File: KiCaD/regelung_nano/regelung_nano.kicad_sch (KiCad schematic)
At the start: 3 parts

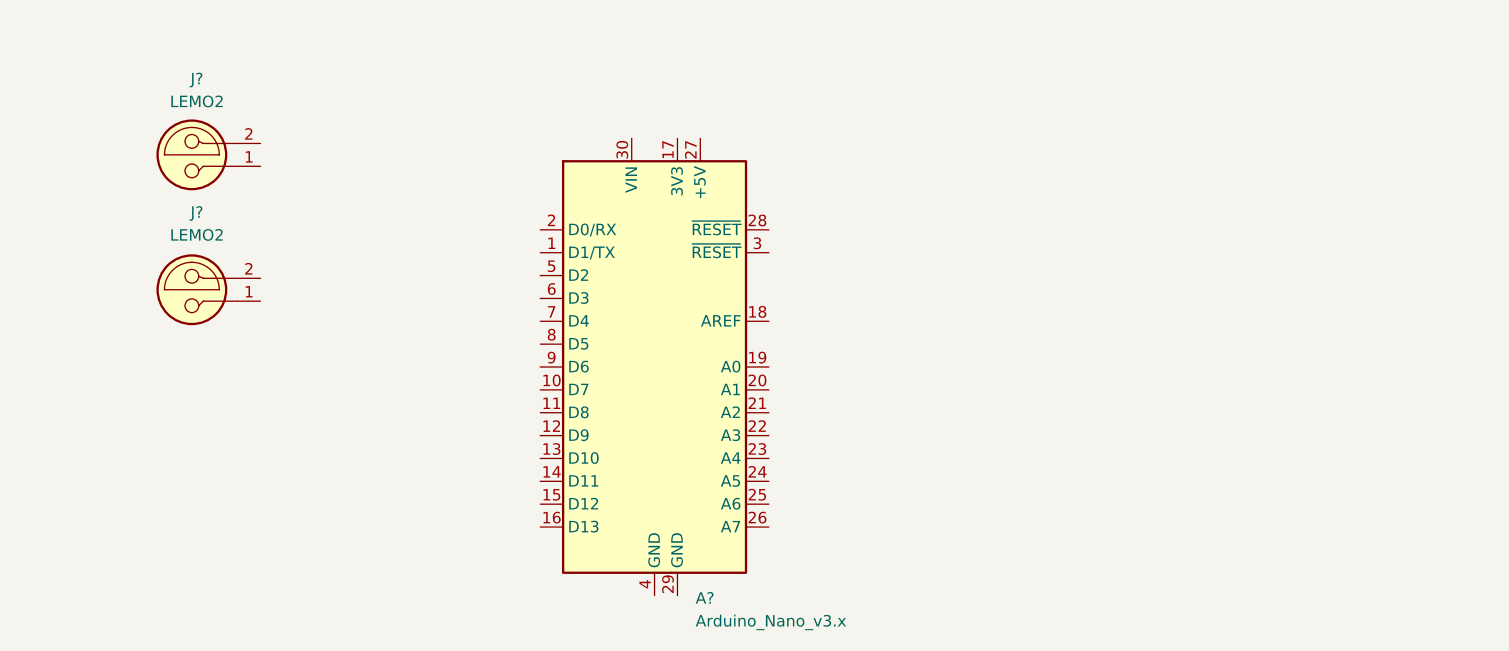
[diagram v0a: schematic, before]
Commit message: ENH: enhance capabilities
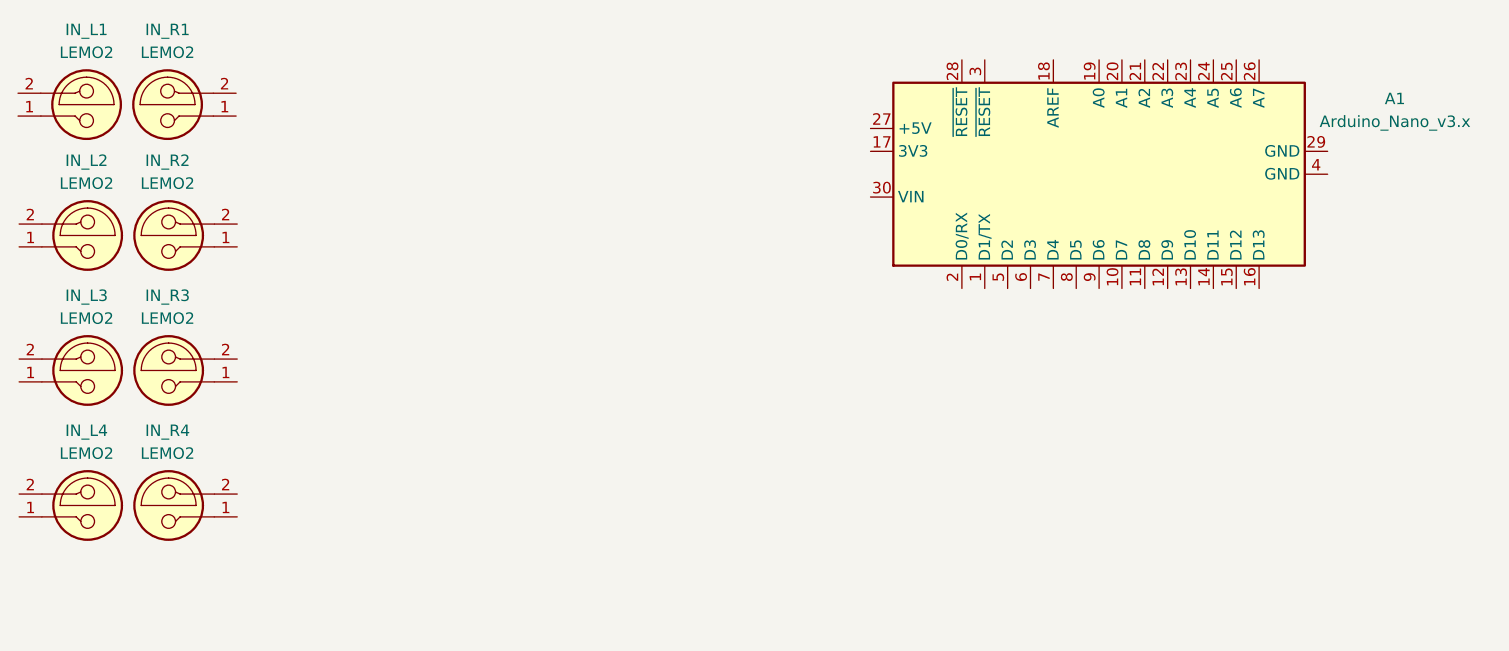
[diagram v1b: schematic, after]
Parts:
- added IN_L1, IN_L2, IN_L3, IN_L4, IN_R1, IN_R4: LEMO2, symbol Connector:LEMO2
- gave numbers to parts that had none: 3
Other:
- moved on the sheet: A1, IN_R2, IN_R3
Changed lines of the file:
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@@
 (kicad_sch (version 20211123) (generator eeschema)
   (paper "A4")
-  (symbol (lib_id "MCU_Module:Arduino_Nano_v3.x") (at 127.6096 61.9252 0) (unit 1)
+  (symbol (lib_id "Connector:LEMO2") (at 73.5 31.5 180) (unit 1)
+    (in_bom yes) (on_board yes)
+    (property "Reference" "IN_R1" (id 0) (at 73.5 24.46 0))
+    (property "Value" "LEMO2" (id 1) (at 73.5 27 0))
+    (property "Footprint" "" (id 2) (at 73.5 32.77 0)
+      (effects (font (size 1.27 1.27)) hide)
+    )
+    (property "Datasheet" " ~" (id 3) (at 73.5 32.77 0)
+      (effects (font (size 1.27 1.27)) hide)
+    )
+    (pin "1")
+    (pin "2")
+  )
+  (symbol (lib_id "Connector:LEMO2") (at 73.62 76.04 180) (unit 1)
+    (in_bom yes) (on_board yes)
+    (property "Reference" "IN_R4" (id 0) (at 73.5 69 0))
+    (property "Value" "LEMO2" (id 1) (at 73.5 71.54 0))
+    (property "Footprint" "" (id 2) (at 73.62 77.31 0)
+      (effects (font (size 1.27 1.27)) hide)
+    )
+    (property "Datasheet" " ~" (id 3) (at 73.62 77.31 0)
+      (effects (font (size 1.27 1.27)) hide)
+    )
+    (pin "1")
+    (pin "2")
+  )
+  (symbol (lib_id "MCU_Module:Arduino_Nano_v3.x") (at 177 40.5 90) (unit 1)
     (in_bom yes) (on_board yes) (fields_autoplaced)
-    (property "Reference" "A?" (id 0) (at 132.169 87.63 0)
-      (effects (font (size 1.27 1.27)) (justify left))
-    )
-    (property "Value" "Arduino_Nano_v3.x" (id 1) (at 132.169 90.17 0)
-      (effects (font (size 1.27 1.27)) (justify left))
-    )
-    (property "Footprint" "Module:Arduino_Nano" (id 2) (at 127.6096 61.9252 0)
+    (property "Reference" "A1" (id 0) (at 209.893 32.1305 90))
+    (property "Value" "Arduino_Nano_v3.x" (id 1) (at 209.893 34.6705 90))
+    (property "Footprint" "Module:Arduino_Nano" (id 2) (at 177 40.5 0)
       (effects (font (size 1.27 1.27) italic) hide)
     )
-    (property "Datasheet" "http://www.mouser.com/pdfdocs/Gravitech_Arduino_Nano3_0.pdf" (id 3) (at 127.6096 61.9252 0)
+    (property "Datasheet" "http://www.mouser.com/pdfdocs/Gravitech_Arduino_Nano3_0.pdf" (id 3) (at 177 40.5 0)
       (effects (font (size 1.27 1.27)) hide)
     )
@@
     (pin "9")
   )
-  (symbol (lib_id "Connector:LEMO2") (at 76.2 37.084 180) (unit 1)
-    (in_bom yes) (on_board yes) (fields_autoplaced)
-    (property "Reference" "J?" (id 0) (at 76.7715 29.9212 0))
-    (property "Value" "LEMO2" (id 1) (at 76.7715 32.4612 0))
-    (property "Footprint" "" (id 2) (at 76.2 38.354 0)
+  (symbol (lib_id "Connector:LEMO2") (at 64.62 61.04 0) (mirror x) (unit 1)
+    (in_bom yes) (on_board yes)
+    (property "Reference" "IN_L3" (id 0) (at 64.5 54 0))
+    (property "Value" "LEMO2" (id 1) (at 64.5 56.54 0))
+    (property "Footprint" "" (id 2) (at 64.62 62.31 0)
       (effects (font (size 1.27 1.27)) hide)
     )
-    (property "Datasheet" " ~" (id 3) (at 76.2 38.354 0)
+    (property "Datasheet" " ~" (id 3) (at 64.62 62.31 0)
       (effects (font (size 1.27 1.27)) hide)
     )
@@
     (pin "2")
   )
-  (symbol (lib_id "Connector:LEMO2") (at 76.2 52.07 180) (unit 1)
-    (in_bom yes) (on_board yes) (fields_autoplaced)
-    (property "Reference" "J?" (id 0) (at 76.7715 44.7548 0))
-    (property "Value" "LEMO2" (id 1) (at 76.7715 47.2948 0))
-    (property "Footprint" "" (id 2) (at 76.2 53.34 0)
+  (symbol (lib_id "Connector:LEMO2") (at 64.62 76.04 0) (mirror x) (unit 1)
+    (in_bom yes) (on_board yes)
+    (property "Reference" "IN_L4" (id 0) (at 64.5 69 0))
+    (property "Value" "LEMO2" (id 1) (at 64.5 71.54 0))
+    (property "Footprint" "" (id 2) (at 64.62 77.31 0)
       (effects (font (size 1.27 1.27)) hide)
     )
-    (property "Datasheet" " ~" (id 3) (at 76.2 53.34 0)
+    (property "Datasheet" " ~" (id 3) (at 64.62 77.31 0)
+      (effects (font (size 1.27 1.27)) hide)
+    )
+    (pin "1")
+    (pin "2")
+  )
+  (symbol (lib_id "Connector:LEMO2") (at 64.62 46.04 0) (mirror x) (unit 1)
+    (in_bom yes) (on_board yes)
+    (property "Reference" "IN_L2" (id 0) (at 64.5 39 0))
+    (property "Value" "LEMO2" (id 1) (at 64.5 41.54 0))
+    (property "Footprint" "" (id 2) (at 64.62 47.31 0)
+      (effects (font (size 1.27 1.27)) hide)
+    )
+    (property "Datasheet" " ~" (id 3) (at 64.62 47.31 0)
+      (effects (font (size 1.27 1.27)) hide)
+    )
+    (pin "1")
+    (pin "2")
+  )
+  (symbol (lib_id "Connector:LEMO2") (at 64.5 31.5 0) (mirror x) (unit 1)
+    (in_bom yes) (on_board yes)
+    (property "Reference" "IN_L1" (id 0) (at 64.5 24.46 0))
+    (property "Value" "LEMO2" (id 1) (at 64.5 27 0))
+    (property "Footprint" "" (id 2) (at 64.5 32.77 0)
+      (effects (font (size 1.27 1.27)) hide)
+    )
+    (property "Datasheet" " ~" (id 3) (at 64.5 32.77 0)
+      (effects (font (size 1.27 1.27)) hide)
+    )
+    (pin "1")
+    (pin "2")
+  )
+  (symbol (lib_id "Connector:LEMO2") (at 73.62 46.04 180) (unit 1)
+    (in_bom yes) (on_board yes)
+    (property "Reference" "IN_R2" (id 0) (at 73.5 39 0))
+    (property "Value" "LEMO2" (id 1) (at 73.5 41.54 0))
+    (property "Footprint" "" (id 2) (at 73.62 47.31 0)
+      (effects (font (size 1.27 1.27)) hide)
+    )
+    (property "Datasheet" " ~" (id 3) (at 73.62 47.31 0)
+      (effects (font (size 1.27 1.27)) hide)
+    )
+    (pin "1")
+    (pin "2")
+  )
+  (symbol (lib_id "Connector:LEMO2") (at 73.62 61.04 180) (unit 1)
+    (in_bom yes) (on_board yes)
+    (property "Reference" "IN_R3" (id 0) (at 73.5 54 0))
+    (property "Value" "LEMO2" (id 1) (at 73.5 56.54 0))
+    (property "Footprint" "" (id 2) (at 73.62 62.31 0)
+      (effects (font (size 1.27 1.27)) hide)
+    )
+    (property "Datasheet" " ~" (id 3) (at 73.62 62.31 0)
       (effects (font (size 1.27 1.27)) hide)
     )
@@
   (symbol_instances
     (path "/45884597-7014-4461-83ee-9975c42b9a53"
-      (reference "A?") (unit 1) (value "Arduino_Nano_v3.x") (footprint "Module:Arduino_Nano")
+      (reference "A1") (unit 1) (value "Arduino_Nano_v3.x") (footprint "Module:Arduino_Nano")
+    )
+    (path "/73a3d458-7c12-4fe9-8c27-9161adf3cdf1"
+      (reference "IN_L1") (unit 1) (value "LEMO2") (footprint "")
+    )
+    (path "/5fb2f18d-4efb-4c56-98b8-d4e9f79e8381"
+      (reference "IN_L2") (unit 1) (value "LEMO2") (footprint "")
+    )
+    (path "/59153f4e-1dc5-46dd-8a20-f2263cd65950"
+      (reference "IN_L3") (unit 1) (value "LEMO2") (footprint "")
+    )
+    (path "/5a90138f-fd69-47b6-87df-f90b07e86699"
+      (reference "IN_L4") (unit 1) (value "LEMO2") (footprint "")
+    )
+    (path "/416dfcbe-1eea-478d-8c11-0e6882ac1192"
+      (reference "IN_R1") (unit 1) (value "LEMO2") (footprint "")
     )
     (path "/9aaf0514-2927-4794-badc-4cc58d8d9fe8"
-      (reference "J?") (unit 1) (value "LEMO2") (footprint "")
+      (reference "IN_R2") (unit 1) (value "LEMO2") (footprint "")
     )
     (path "/f2c46314-84ea-4f10-8742-a38a82344d5e"
-      (reference "J?") (unit 1) (value "LEMO2") (footprint "")
+      (reference "IN_R3") (unit 1) (value "LEMO2") (footprint "")
+    )
+    (path "/446bf39e-f653-4e79-b238-d1778bb60fa7"
+      (reference "IN_R4") (unit 1) (value "LEMO2") (footprint "")
     )
   )
